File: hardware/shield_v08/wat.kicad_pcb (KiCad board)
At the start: 2 copper layers, 40 parts, among them P101 24VOL, P102 CAUDAL_1, P103 V_IN, P104 PRESION_1, P105 INTENSIDAD_1, P106 18b20, P107 INTENSIDAD_2, P108 15VOL, P109 LCD_I2C, P110 ARD_DI_06, P111 ARD_ALI_04, P112 ARD_AN_I2C, U101 ESP-12, U102 Recom-rd, U103 RO-1224S, U104 LM1117, U105 mp-1584, U106 NANO

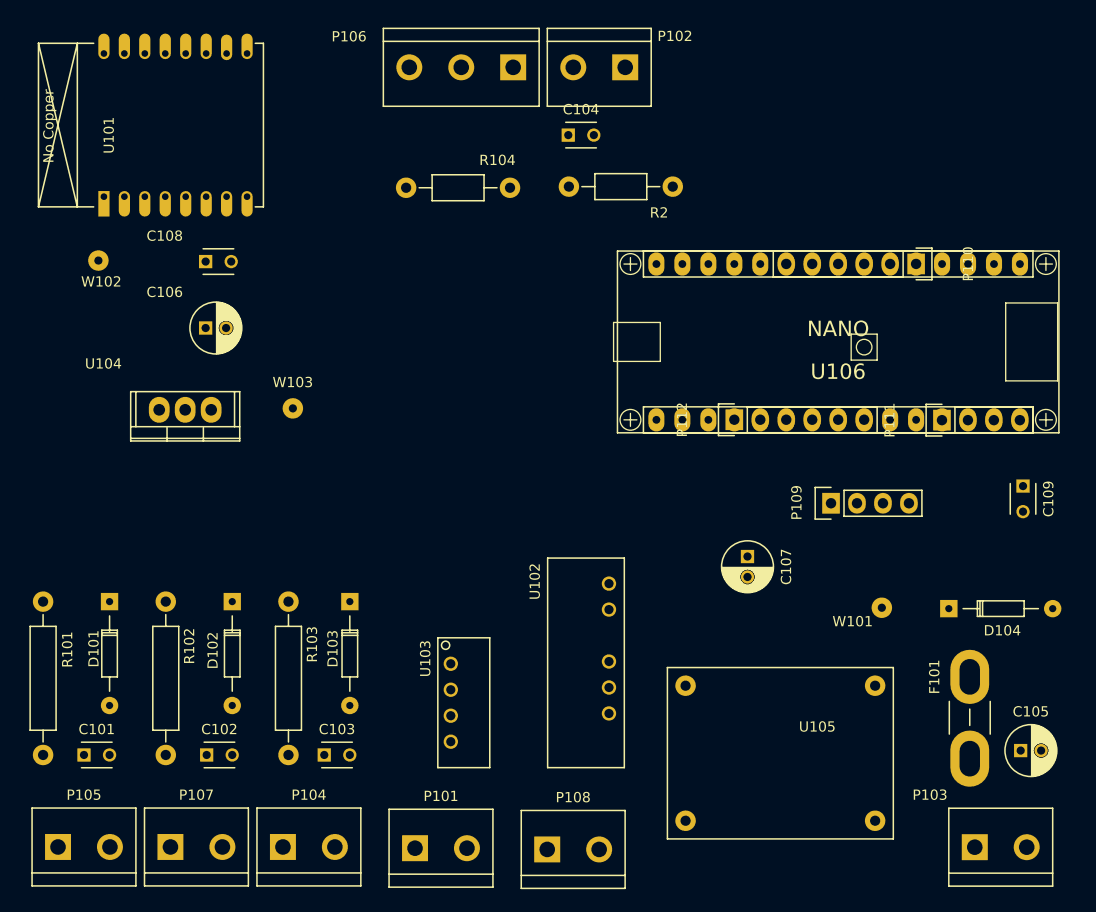
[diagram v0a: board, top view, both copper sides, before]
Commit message: [pcb]avance version 3
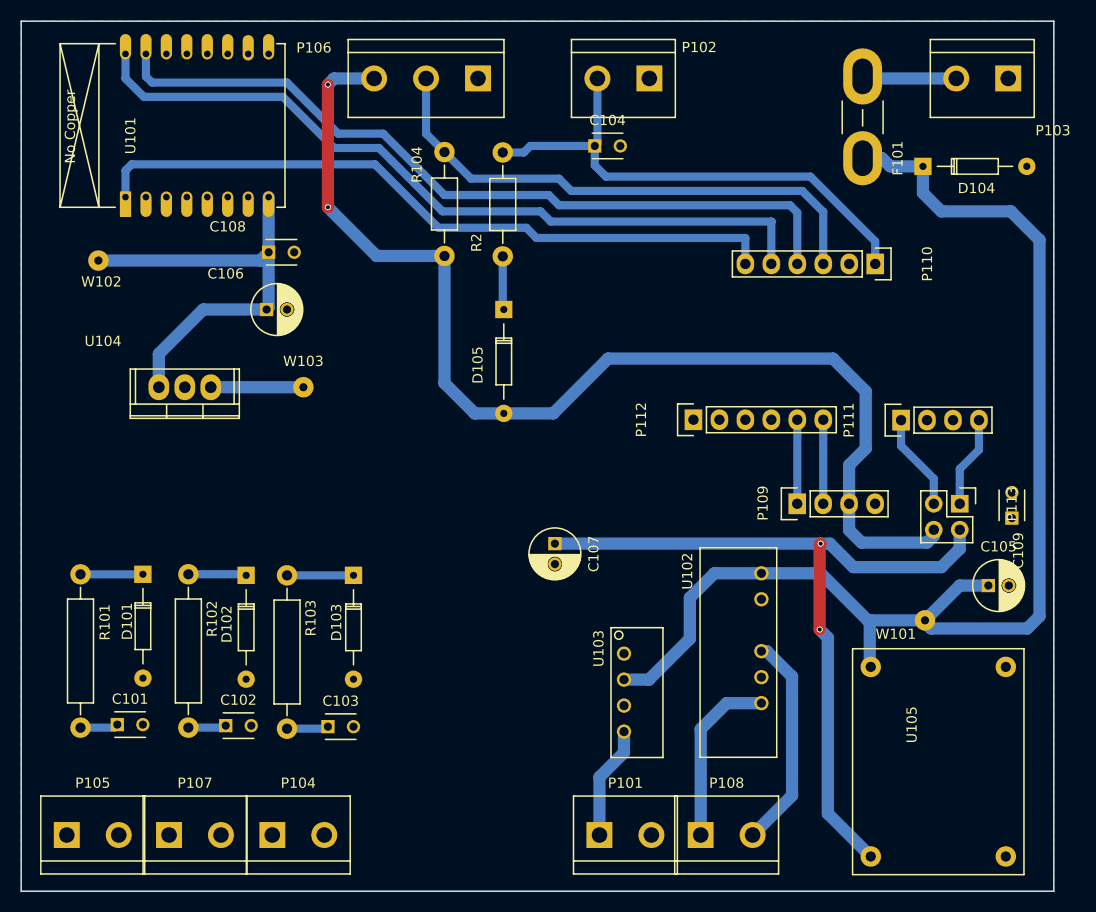
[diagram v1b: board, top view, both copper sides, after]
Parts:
- removed U106: NANO, oscar_libreria_huellas:arduino_nano
- added D105: 1N4007, Diodes_ThroughHole:Diode_DO-35_SOD27_Horizontal_RM10, F.Cu at (101.0, 71.0)
- added P113: CONN_02X02, Pin_Headers:Pin_Header_Straight_2x02, F.Cu at (145.6, 90.0)
- moved P103 75.2 mm to (147.8, 48.4), turned to 180 degrees
- moved F101 59.7 mm to (136.1, 52.2), turned to 270 degrees
- moved D104 43.3 mm to (142.0, 57.0)
- moved C107 18.9 mm to (106.0, 93.9)
- moved P101 18.1 mm to (112.9, 122.4)
- moved R2 18.0 mm to (100.9, 65.8), turned to 90 degrees
- moved U103 17.0 mm to (115.3, 107.2)
- moved C105 16.4 mm to (148.4, 98.0)
- moved U105 15.3 mm to (143.5, 115.1), turned to 270 degrees
- moved P108 15.1 mm to (122.8, 122.4)
- moved U102 14.9 mm to (126.2, 96.8)
- moved R104 7.30 mm to (95.2, 55.6), turned to 270 degrees
- moved C106 6.23 mm to (77.8, 71.0)
- moved C108 6.23 mm to (78.0, 65.4)
- moved R101 4.53 mm to (59.6, 96.9)
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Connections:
- P103 pad 1: Net-(F101-Pad1) -> GND
- P103 pad 2: GND -> Net-(F101-Pad1)
- P111 pad 1: /Vpc_5V -> Net-(P111-Pad1)
- P111 pad 4: /Var_8V -> Net-(P111-Pad4)
- R2 pad 1: /Vpc_5V -> Net-(D105-Pad1)
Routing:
- net /Vin_12V: track 0.00 -> 121.7 mm
- net /Vpc_5V: track 0.00 -> 112.5 mm, vias 0 -> 2
- net /Var_8V: track 0.00 -> 84.9 mm, vias 0 -> 2
- net /e_rx: track 0.00 -> 76.5 mm
- net /e_tx: track 0.00 -> 75.6 mm
- net /e_rst: track 0.00 -> 69.0 mm
- net /18b20: track 0.00 -> 52.5 mm
- net /caudal_1: track 0.00 -> 50.6 mm
- net /Ves_3V3: track 0.00 -> 43.7 mm
- net Net-(P108-Pad2): track 0.00 -> 21.1 mm
- net Net-(P108-Pad1): track 0.00 -> 17.4 mm
- net Net-(P101-Pad1): track 0.00 -> 11.1 mm
- net Net-(P111-Pad1): track 0.00 -> 9.51 mm
- net Net-(F101-Pad1): track 0.00 -> 9.24 mm
- net Net-(P111-Pad4): track 0.00 -> 8.96 mm
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- added copper zone on B.Cu, net GND
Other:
- board outline added: 101 x 85.1 mm
